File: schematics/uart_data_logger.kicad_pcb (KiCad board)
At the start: 2 copper layers, 10 parts, among them J1 Micro_SD_Card, SW1 Start/Stop, U1 CH32V003F4P6

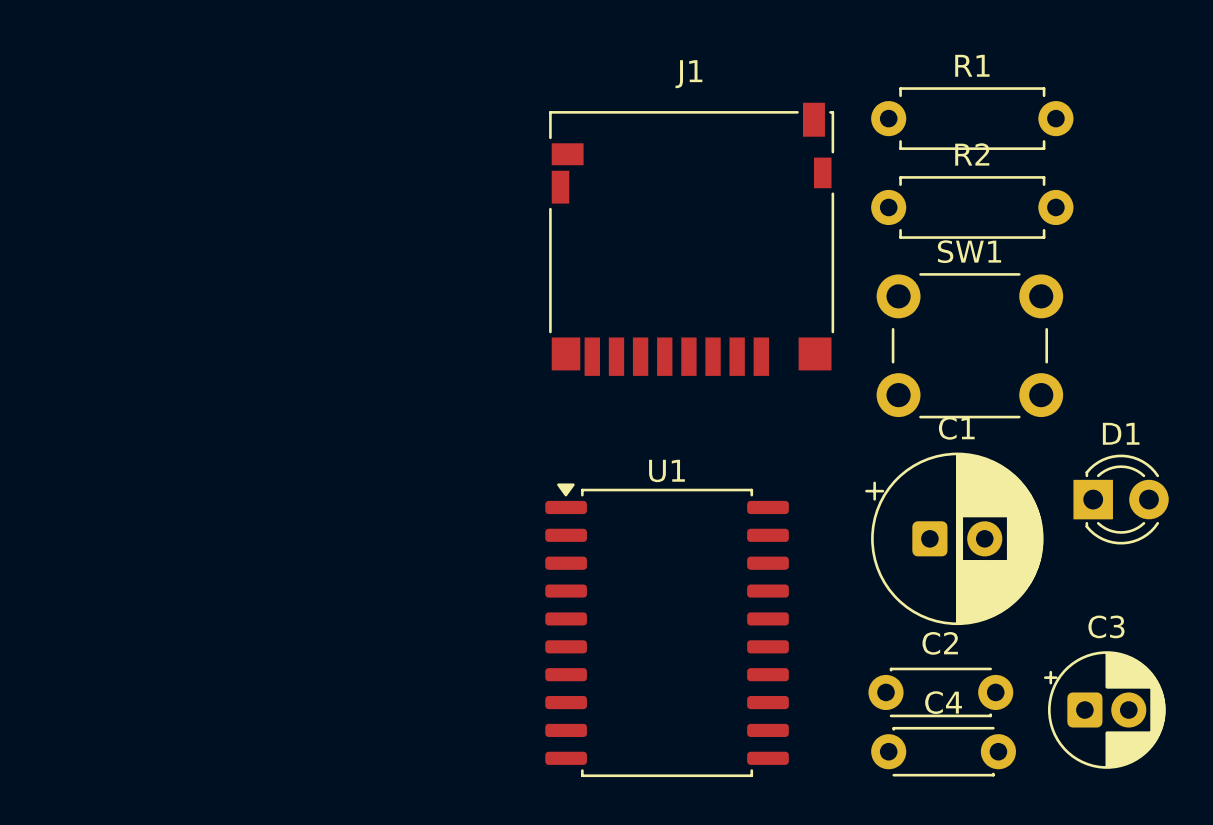
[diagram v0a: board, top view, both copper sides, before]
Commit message: updated schematics/layout.
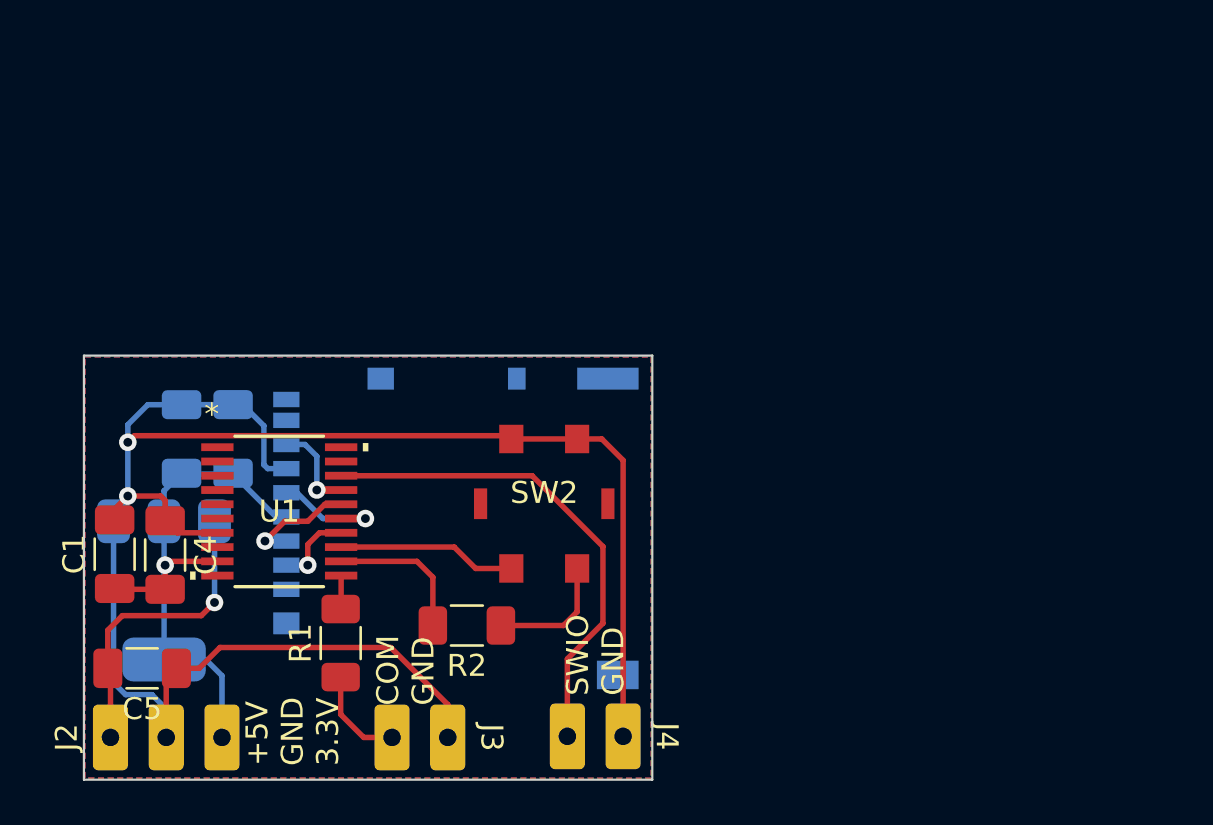
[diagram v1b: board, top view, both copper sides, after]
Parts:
- removed D1: STATUS, LED_THT:LED_D3.0mm
- removed SW1: Start/Stop, Button_Switch_THT:SW_PUSH_6mm_H4.3mm
- added C5: 10uF, Capacitor_SMD:C_1206_3216Metric_Pad1.33x1.80mm_HandSolder, F.Cu at (91.6, 103.4)
- added J2: Conn_01x03, swk:1x03_THT_P2.54mm, F.Cu at (90.2, 106.5)
- added J3: Conn_01x02, swk:1x02_THT_P2.54mm, F.Cu at (105.5, 106.5)
- added J4: Conn_01x02, swk:1x02_THT_P2.54mm, F.Cu at (113.5, 106.5)
- added SW2: SW_Push_LED, swk:SW_Push_LED_AK104238, F.Cu at (109.9, 95.9)
- added U3: AZ1117CH-3.3TRG1, Package_TO_SOT_SMD:SOT-223-3_TabPin2, B.Cu at (92.6, 99.8)
- C1: value 220uf -> 100uF; footprint Capacitor_THT:CP_Radial_D7.5mm_P2.50mm -> Capacitor_SMD:C_1206_3216Metric_Pad1.33x1.80mm_HandSolder
- C2: footprint Capacitor_THT:C_Disc_D4.3mm_W1.9mm_P5.00mm -> Capacitor_SMD:C_1206_3216Metric_Pad1.33x1.80mm_HandSolder; moved to B.Cu
- C3: footprint Capacitor_THT:CP_Radial_D5.0mm_P2.00mm -> Capacitor_SMD:C_1206_3216Metric_Pad1.33x1.80mm_HandSolder; moved to B.Cu
- C4: footprint Capacitor_THT:C_Disc_D4.3mm_W1.9mm_P5.00mm -> Capacitor_SMD:C_1206_3216Metric_Pad1.33x1.80mm_HandSolder
- J1: footprint Connector_Card:microSD_HC_Hirose_DM3D-SF -> Connector_Card:microSD_HC_Hirose_DM3AT-SF-PEJM5; moved to B.Cu
- R1, R2: footprint Resistor_THT:R_Axial_DIN0207_L6.3mm_D2.5mm_P7.62mm_Horizontal -> Resistor_SMD:R_1206_3216Metric_Pad1.30x1.75mm_HandSolder
- U1: footprint Package_SO:SOP-20_7.5x12.8mm_P1.27mm -> swk:TSSOP20
- moved C3 43.0 mm to (93.4, 92.9), turned to 90 degrees
- moved C1 37.2 mm to (90.3, 98.2), turned to 90 degrees
- moved R1 34.6 mm to (100.7, 102.2), turned to 90 degrees
- moved C4 34.2 mm to (92.7, 98.2), turned to -90 degrees
- moved C2 31.9 mm to (95.7, 92.9), turned to -90 degrees
- moved R2 27.1 mm to (106.4, 101.5), turned to 180 degrees
- moved U1 18.5 mm to (97.8, 96.2)
- moved J1 17.0 mm to (105.9, 97.0), turned to -90 degrees
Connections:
- J1 pad 10: (no net) -> unconnected-(J1-DET_A-Pad10)
- J1 pad 9: (no net) -> unconnected-(J1-DET_B-Pad9)
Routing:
- net GND: track 0.00 -> 87.4 mm, vias 0 -> 2
- net +3.3V: track 0.00 -> 26.1 mm, vias 0 -> 1
- net PRG_SWIO: track 0.00 -> 22.6 mm
- net Net-(J2-Pin_1): track 0.00 -> 14.0 mm, vias 0 -> 1
- net Net-(U1-PC3): track 0.00 -> 8.16 mm
- net Net-(U1-PC2): track 0.00 -> 6.68 mm
- net Net-(R2-Pad1): track 0.00 -> 5.71 mm
- net /SCK: track 0.00 -> 5.19 mm, vias 0 -> 1
- net /MOSI: track 0.00 -> 5.14 mm, vias 0 -> 1
- net COMM_Rx: track 0.00 -> 4.47 mm
- net /MISO: track 0.00 -> 4.25 mm, vias 0 -> 1
- net /CS: track 0.00 -> 3.66 mm, vias 0 -> 1
- net Net-(U1-PC1): track 0.00 -> 1.53 mm
- added copper zone on B.Cu, net GND
- added copper zone on F.Cu, net GND
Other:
- board outline added: 25.9 x 19.3 mm
- board text added: "+5V GND 3.3V"
- board text added: "COM GND"
- board text added: "SWIO GND"
